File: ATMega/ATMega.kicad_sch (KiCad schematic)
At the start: 7 parts

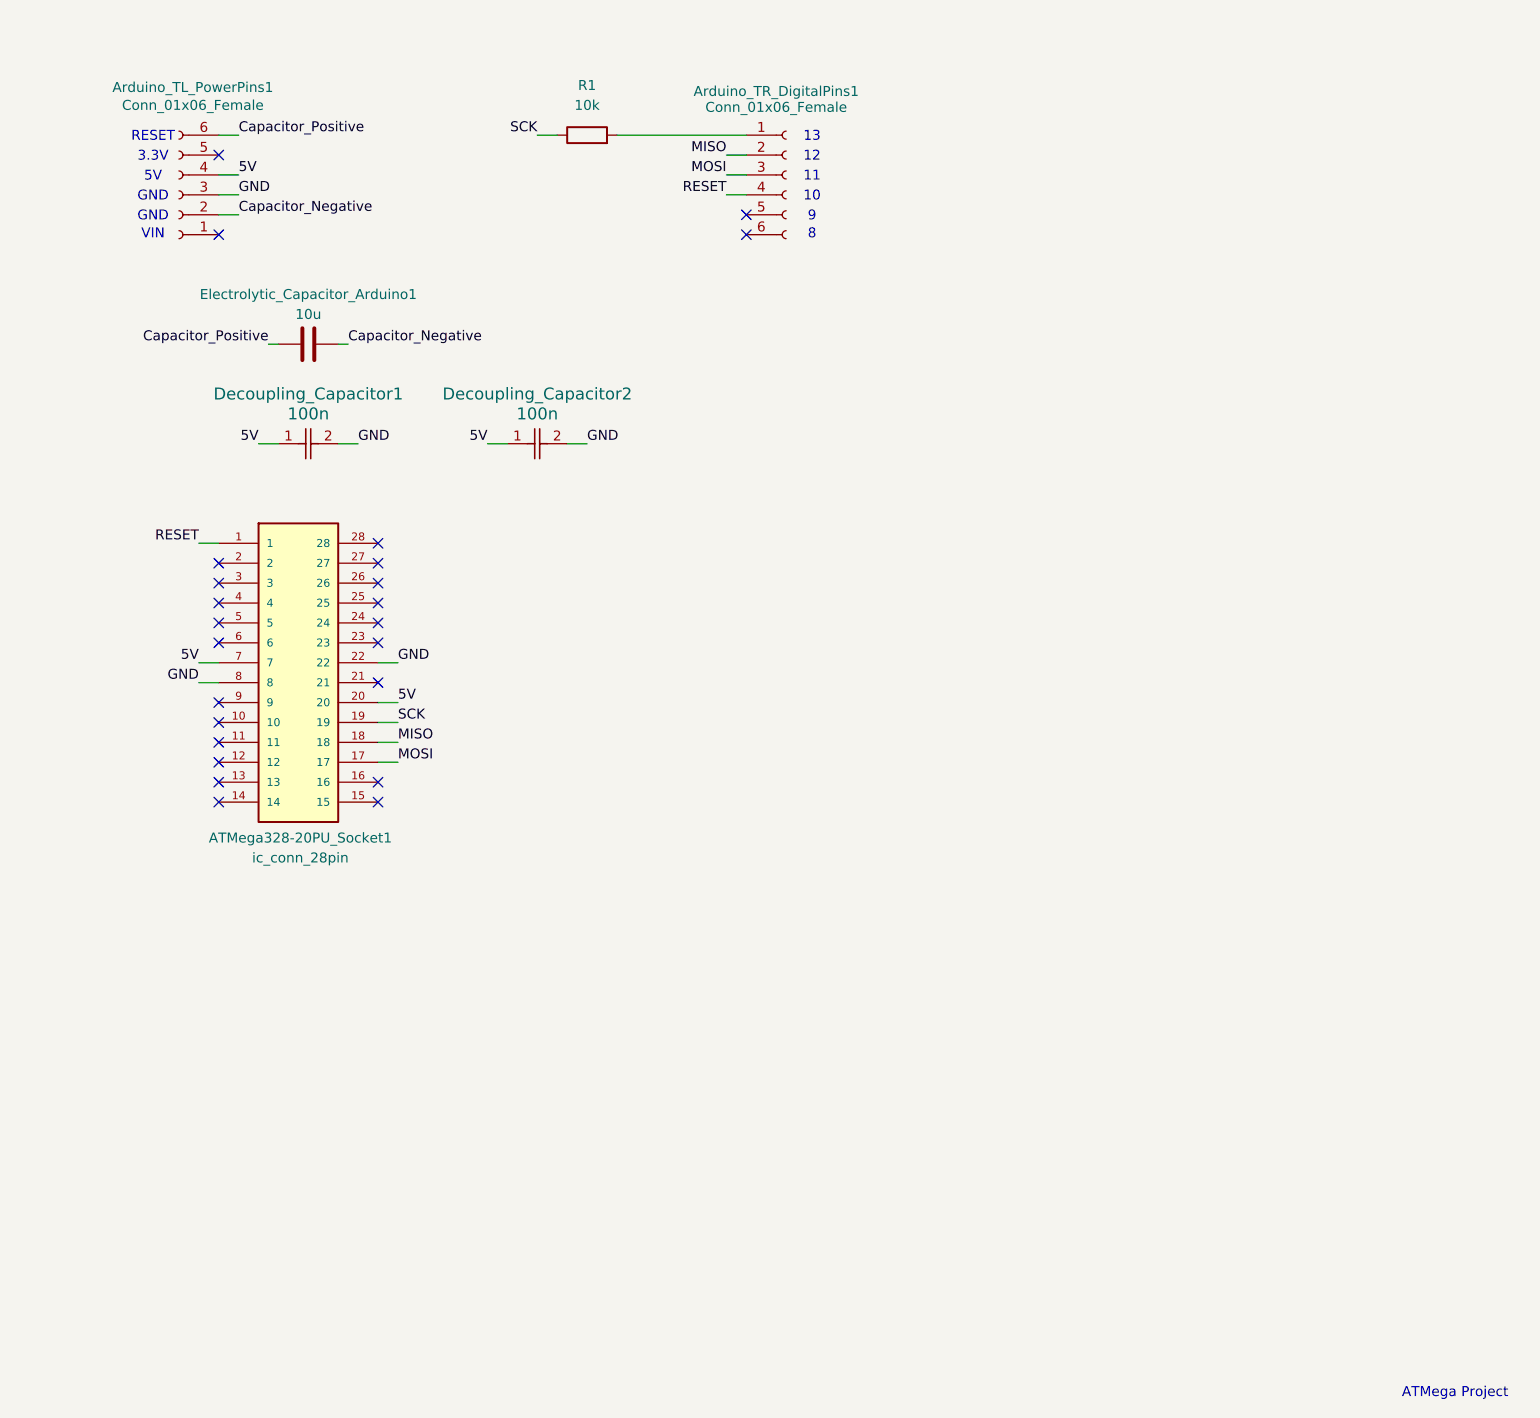
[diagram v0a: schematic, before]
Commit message: ATMega adjust
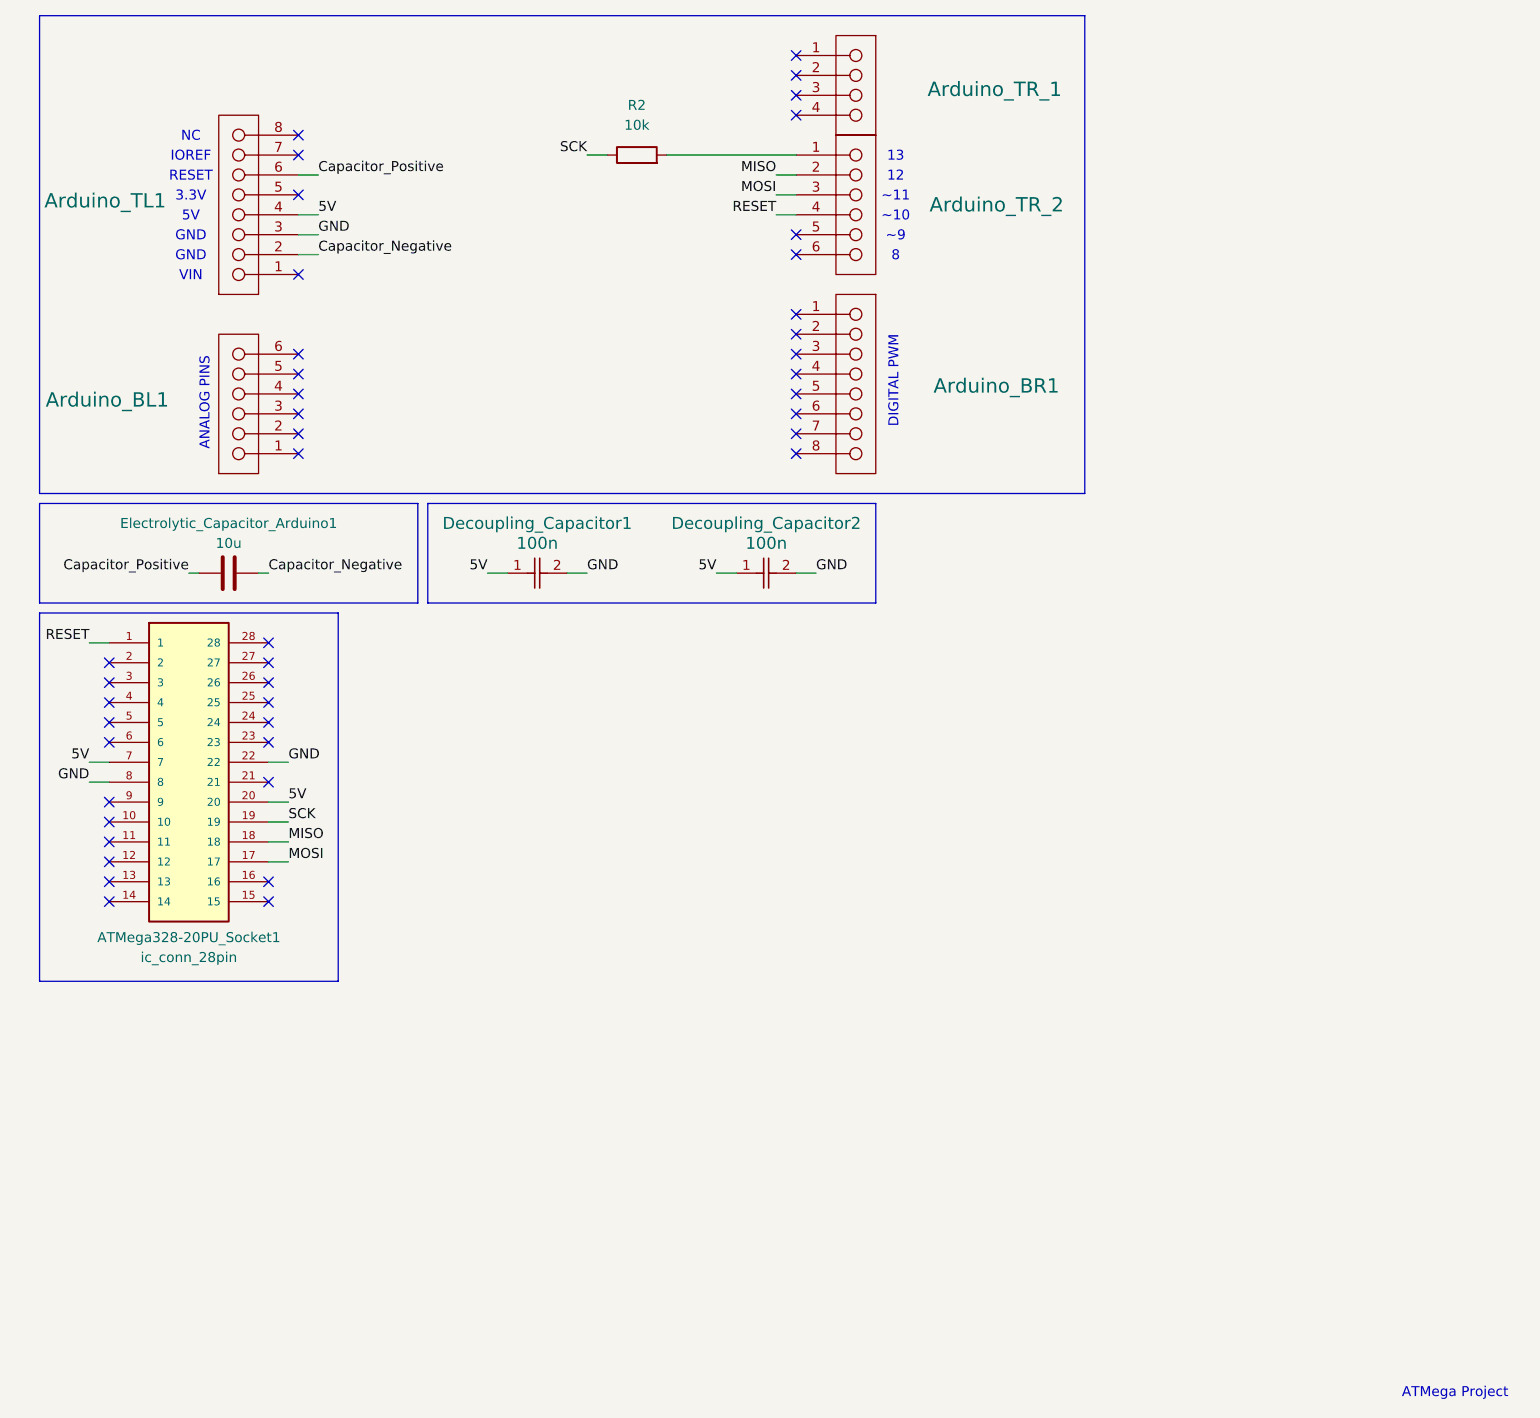
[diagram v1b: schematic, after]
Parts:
- removed Arduino_TL_PowerPins1, Arduino_TR_DigitalPins1: Conn_01x06_Female, rsx_headers:PinSocket_1x06_P2.54mm_Vertical, symbol rsx_header:Conn_01x06_Female
- removed R1: 10k, rsx_resistors:R_0603_1608Metric, symbol rsx_Resistors:10k
- added Arduino_BL1, Arduino_TR_2: header_1x6_arduino, Connector_PinHeader_2.54mm:PinHeader_1x06_P2.54mm_Vertical, symbol rsx_header:header_1x6_arduino
- added Arduino_BR1, Arduino_TL1: header_1x8_arduino, Connector_PinHeader_2.54mm:PinHeader_1x08_P2.54mm_Vertical, symbol rsx_header:header_1x8_arduino
- added Arduino_TR_1: header_1x4_arduino, Connector_PinHeader_2.54mm:PinHeader_1x04_P2.54mm_Vertical, symbol rsx_header:header_1x4_arduino
- added R2: 10k, rsx_resistors:R_0603_1608Metric, symbol rsx_Resistors:10k
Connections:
- net 5V: now also Arduino_TL1.4
- net Capacitor_Negative: now also Arduino_TL1.2
- net Capacitor_Positive: now also Arduino_TL1.6
- net GND: now also Arduino_TL1.3
- net MISO: now also Arduino_TR_2.2
- net MOSI: now also Arduino_TR_2.3
- net RESET: now also Arduino_TR_2.4
- net SCK: now also R2.1
- new net: Arduino_TR_2.1, R2.2
- no-connect marks 24 -> 44
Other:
- note added: "ANALOG PINS"
- note added: "DIGITAL PWM"
- note added: "IOREF"
- note added: "NC"
- note added: "~10"
- note added: "~11"
- note added: "~9"
- note removed: "10"
- note removed: "11"
- note removed: "9"
